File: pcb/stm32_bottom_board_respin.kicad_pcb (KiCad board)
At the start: 2 copper layers, 100 x 70 mm, 91 parts, among them J1 48V_SRC, J10 FCC_B2B, J11 SSR2_CTRL, J12 POWER, J13 PMS7003S_CONN, J14 MAINBOARD_CONN, J2 WS2812_CTRL, J3 FAN_CTRL, J4 SSR_OUTPUT, J5 PURFUME_CTRL, J6 Conn_01x14, J7 Conn_01x12, J8 Conn_01x15, J9 PCB_UART, Q1 2N3904(1AM), Q2 SS9013_J3, Q3 2N3904(1AM), Q4 2N3904(1AM), SW1 SW_Push, U1 74AHCT1G125, U2 OMRON-G3MB-202P, U3 STM32F103C8T6, U4 AMS1117-3.3, U5 SP3232EEN, U6 OMRON-G3MB-202P, U7 waveshare-swd-pinsocket, Y1 O8M, Y2 O_EPSON_32.768K

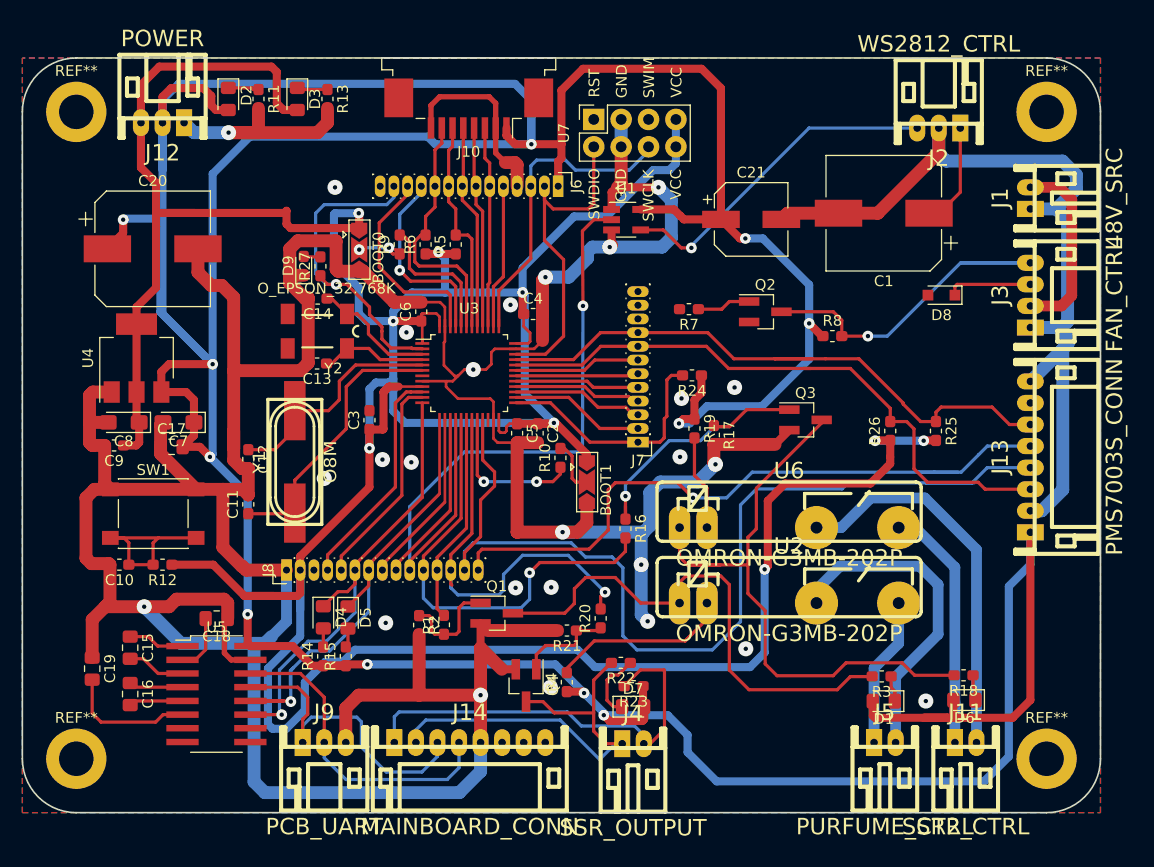
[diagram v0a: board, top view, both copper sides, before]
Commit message: update,
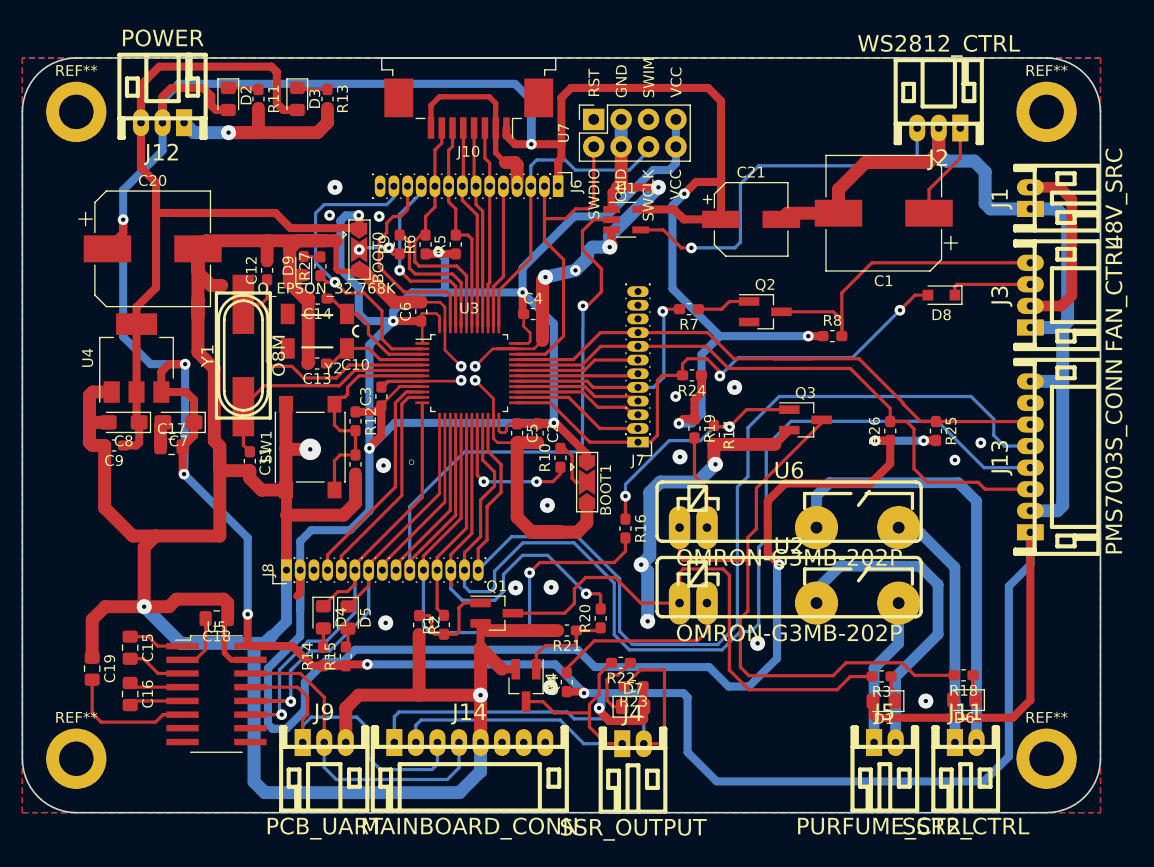
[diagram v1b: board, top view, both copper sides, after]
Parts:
- moved C10 23.8 mm to (60.9, 67.7), turned to 270 degrees
- moved R12 22.3 mm to (60.9, 63.7), turned to 270 degrees
- moved C12 17.6 mm to (52.7, 49.7), turned to 90 degrees
- moved SW1 15.8 mm to (56.7, 66.1), turned to 90 degrees
- moved Y1 11.0 mm to (50.5, 57.6)
- moved C11 4.00 mm to (51.1, 67.4), turned to 270 degrees
- moved C3 2.45 mm to (63.3, 61.4)
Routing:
- net +5V: track 442.3 -> 375.3 mm
- net STM32_PMS7003S_RXD: track 63.9 -> 97.3 mm, vias 1 -> 0
- net STM32_FAN_RPM: track 22.5 -> 50.6 mm, vias 0 -> 2
- net GND: track 503.5 -> 521.9 mm, vias 26 -> 32
- net +3V3: track 365.4 -> 353.1 mm
- net STM32_FAN_PWM_OUTPUT: track 11.6 -> 22.2 mm, vias 0 -> 1
- net /SSR_CH2_OUTPUT1: track 35.9 -> 41.4 mm
- net /STM32_CORE/OSCIN: track 21.4 -> 26.8 mm
- net STM32_SSR2_OUTPUT: track 41.9 -> 46.7 mm
- net /WS2812_PWM_TERMINAL: track 31.1 -> 35.7 mm
- net /FAN_PWM_OUTPUT: track 34.1 -> 30.1 mm, vias 1 -> 0
- net /STM32_CORE/RESET: track 16.8 -> 20.9 mm
- net STM32_PMS7003S_TXD: track 95.7 -> 99.2 mm
- net /STM32_CORE/OSCOUT: track 25.7 -> 22.4 mm
- net STM32_PMS7003S_SET: track 57.8 -> 55.8 mm
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
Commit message: update,
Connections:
- J14 pad 1: /SSR-25-DA_P -> GND
- J14 pad 2: /SSR-25-DA_N -> /SSR-25-DA_P
- J14 pad 3: /IONAIR_RX -> /SSR-25-DA_N
- J14 pad 4: /IONAIR_TX -> /IONAIR_RX
- J14 pad 5: GND -> /IONAIR_TX
- J14 pad 6: Net-(J14-Pad6) -> PCB1_ALARM_COM
- J14 pad 8: Net-(J14-Pad8) -> +5V
- J8 pad 9: /STM32_CORE/PA5 -> PCB1_ALARM_COM
- U3 pad 15: /STM32_CORE/PA5 -> PCB1_ALARM_COM
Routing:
- net PCB1_ALARM_COM: track 0.00 -> 16.0 mm
- net /STM32_CORE/PA5: track 16.0 -> 0.00 mm
